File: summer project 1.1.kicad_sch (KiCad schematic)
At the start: 1 part, among them U3 LM5050-1_mod2

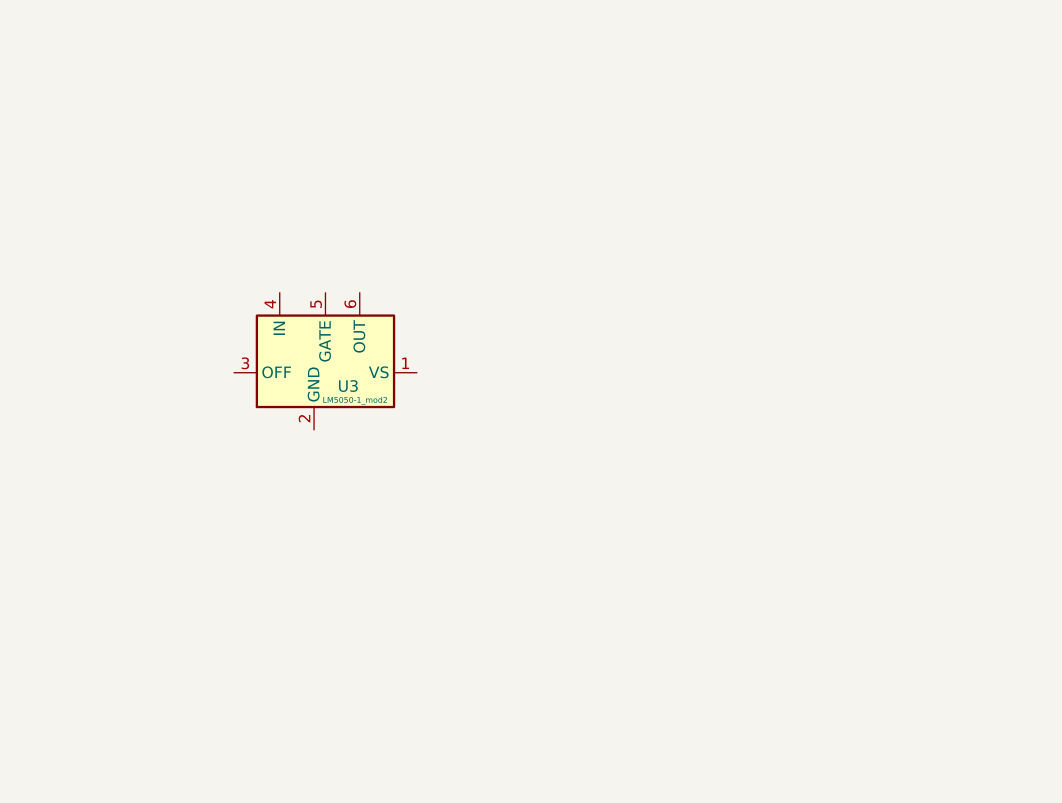
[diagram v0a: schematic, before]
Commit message: Schematic Design Completed
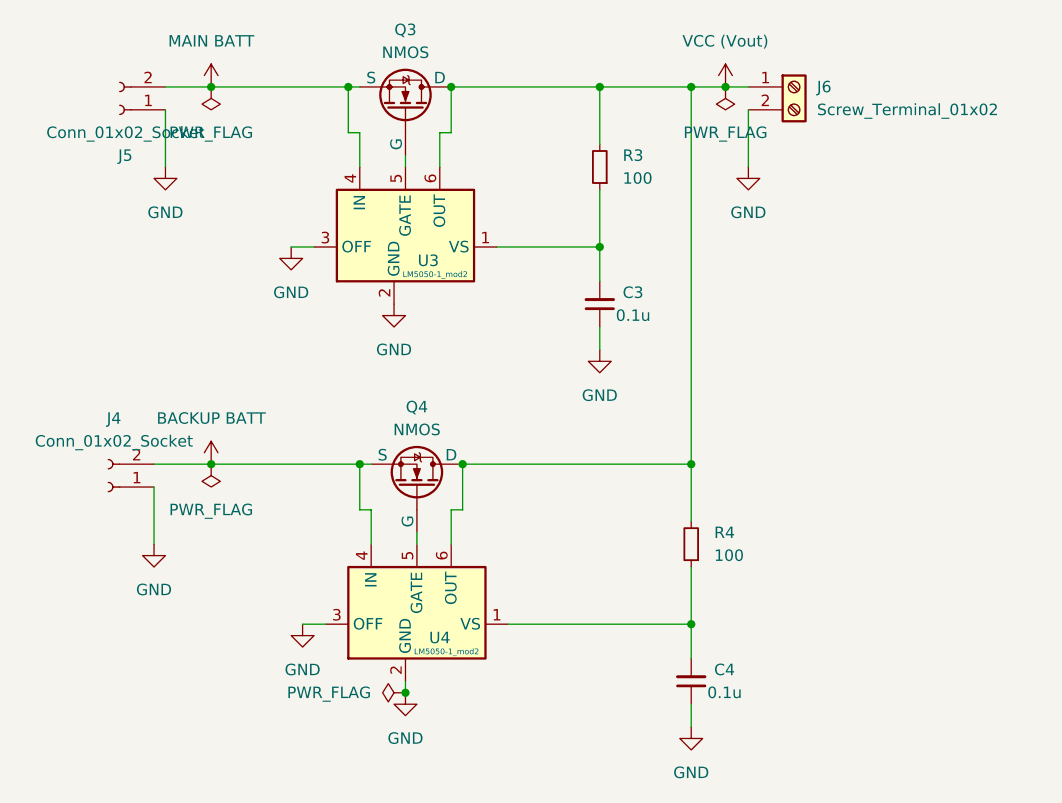
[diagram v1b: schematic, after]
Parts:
- added C3, C4: 0.1u, Capacitor_SMD:C_0603_1608Metric, symbol Device:C_Small
- added J4, J5: Conn_01x02_Socket, Connector_AMASS:AMASS_XT30U-F_1x02_P5.0mm_Vertical, symbol Connector:Conn_01x02_Socket
- added J6: Screw_Terminal_01x02, TerminalBlock_Phoenix:TerminalBlock_Phoenix_MKDS-3-2-5.08_1x02_P5.08mm_Horizontal, symbol Connector:Screw_Terminal_01x02
- added Q3, Q4: NMOS, Package_TO_SOT_SMD:TO-252-3_TabPin2, symbol Simulation_SPICE:NMOS
- added R3, R4: 100, Resistor_SMD:R_0603_1608Metric, symbol Device:R_Small
- added U4: LM5050-1_mod2, Package_TO_SOT_SMD:TSOT-23-6, symbol smp 1:LM5050-1_mod2
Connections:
- net at U3.1 (VS): now also C3.2, R3.1
- net GND: now reaches U3.2 (GND)
- net GND: now also U3.3 (OFF), C3.1, C4.1, J4.1 (Pin_1), J5.1 (Pin_1), J6.2 (Pin_2), U4.2 (GND), U4.3 (OFF)
- net MAIN BATT: now reaches U3.4 (IN)
- net MAIN BATT: now also J5.2 (Pin_2), Q3.3 (S)
- net at U3.5 (GATE): now also Q3.2 (G)
- net VCC (Vout): now reaches U3.6 (OUT)
- net VCC (Vout): now also J6.1 (Pin_1), Q3.1 (D), Q4.1 (D), R3.2, R4.2, U4.6 (OUT)
- new net: C4.2, R4.1, U4.1 (VS)
- new net: Q4.2 (G), U4.5 (GATE)
- new net BACKUP BATT: J4.2 (Pin_2), Q4.3 (S), U4.4 (IN)
